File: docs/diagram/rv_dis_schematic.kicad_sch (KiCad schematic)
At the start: 1 part

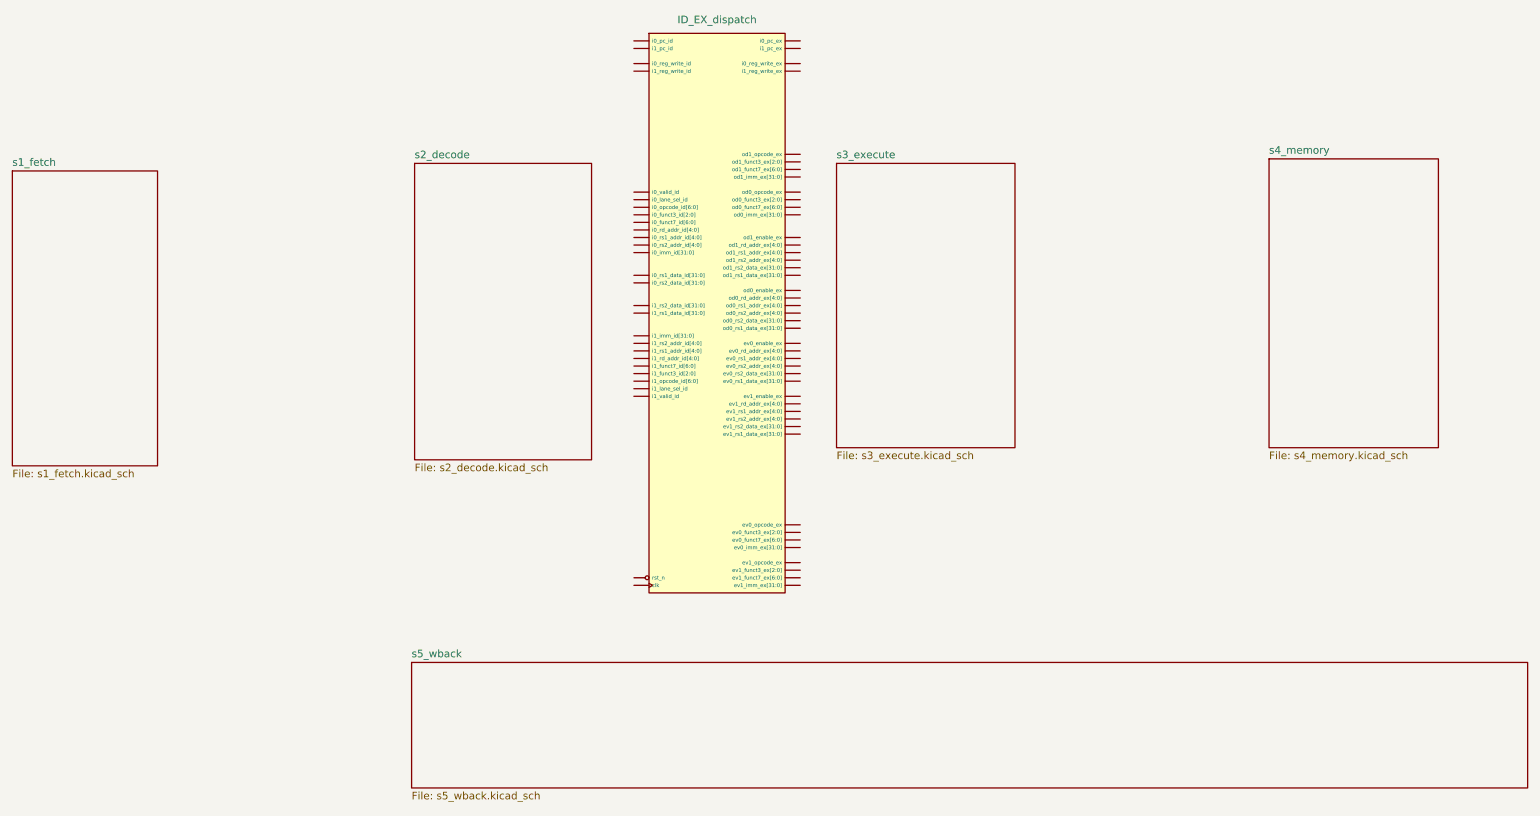
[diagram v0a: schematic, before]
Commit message: push
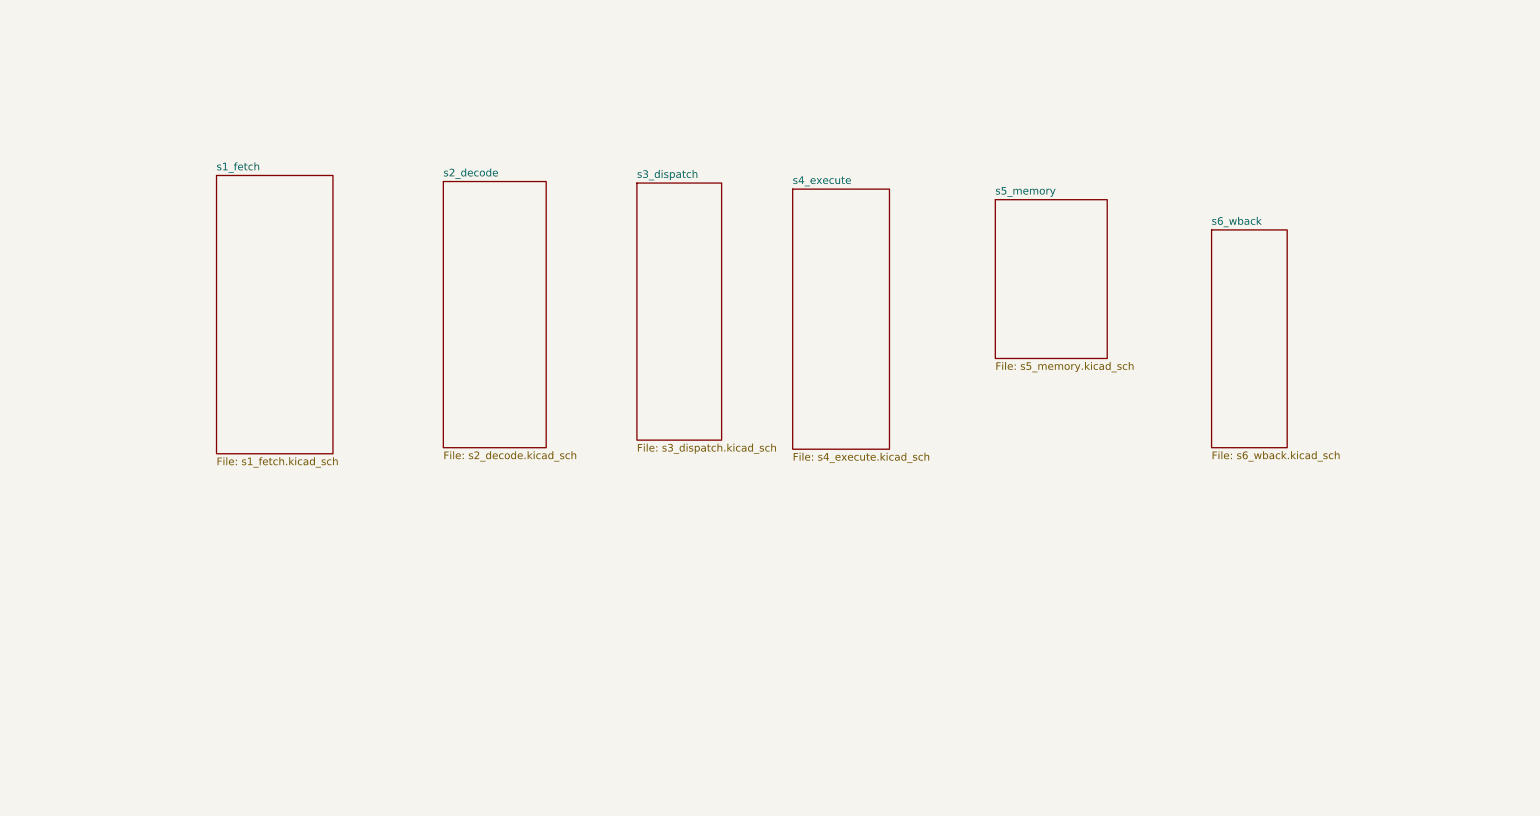
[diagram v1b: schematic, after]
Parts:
- removed ID_EX_dispatch: ~, symbol RV-DIS:ID_EX_dispatch
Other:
- sheet s3_execute renamed s4_execute
- sheet s4_memory renamed s5_memory
- removed sheet s5_wback
- added sheet s3_dispatch (s3_dispatch.kicad_sch)
- added sheet s6_wback (s6_wback.kicad_sch)
- sheet s4_execute: file s3_execute.kicad_sch -> s4_execute.kicad_sch
- sheet s5_memory: file s4_memory.kicad_sch -> s5_memory.kicad_sch
